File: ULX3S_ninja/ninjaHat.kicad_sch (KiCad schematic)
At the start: 14 parts, among them J1 DVI-HX-107DIP, P1 ULX3S connector (JP1)

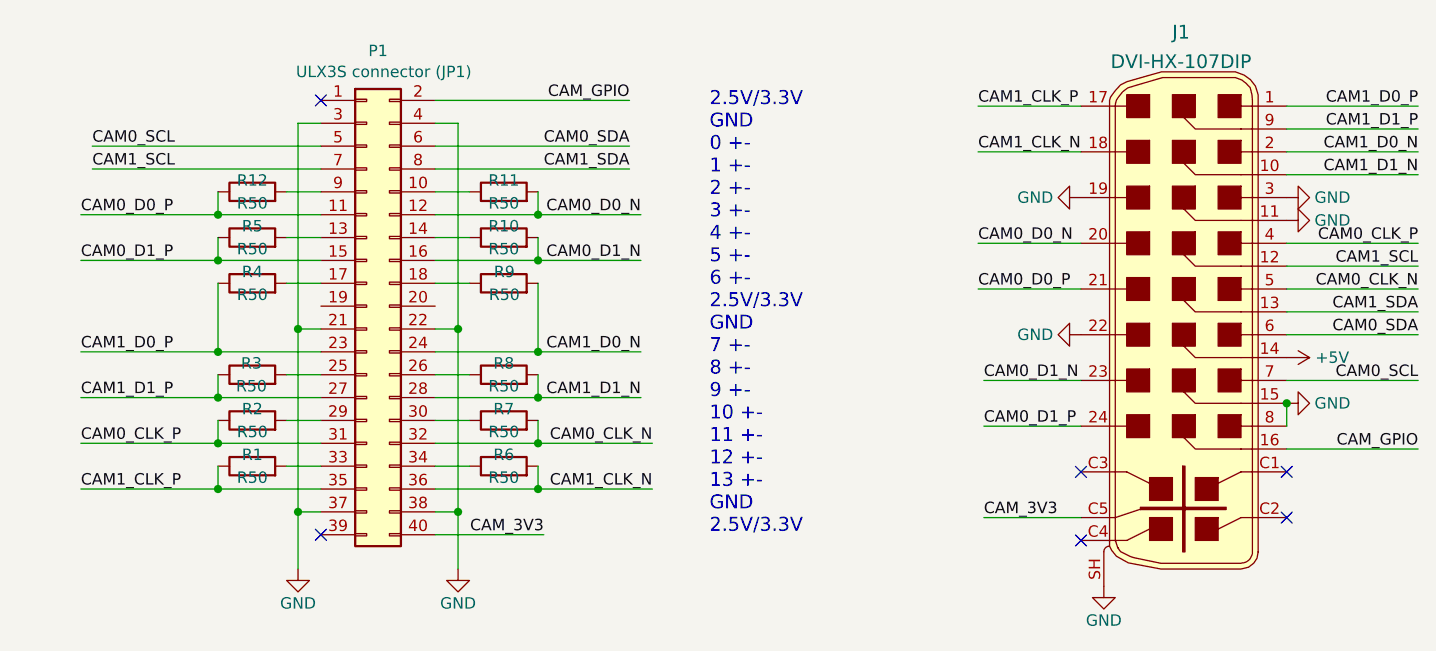
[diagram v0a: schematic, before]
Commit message: Changed circuit
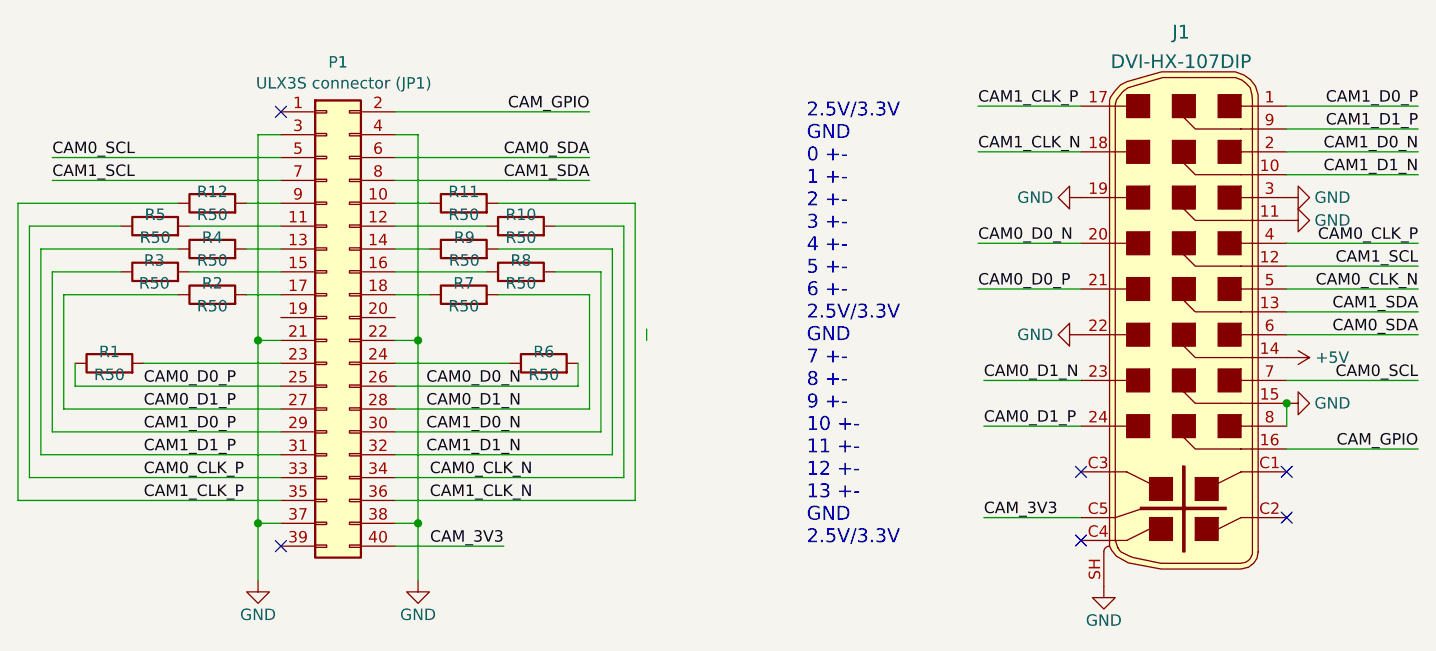
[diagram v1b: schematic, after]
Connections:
- net CAM0_CLK_N: now also P1.34 (Pin_34), R10.2; no longer P1.32 (Pin_32), R7.2
- net CAM0_CLK_P: now also P1.33 (Pin_33), R5.1; no longer P1.31 (Pin_31), R2.1
- net CAM0_D0_N: now also P1.26 (Pin_26), R6.2; no longer P1.12 (Pin_12), R11.2
- net CAM0_D0_P: now also P1.25 (Pin_25), R1.1; no longer P1.11 (Pin_11), R12.1
- net CAM0_D1_N: now also P1.28 (Pin_28), R7.2; no longer P1.16 (Pin_16), R10.2
- net CAM0_D1_P: now also P1.27 (Pin_27), R2.1; no longer P1.15 (Pin_15), R5.1
- net CAM1_CLK_N: now also R11.2; no longer R6.2
- net CAM1_CLK_P: now also R12.1; no longer R1.1
- net CAM1_D0_N: now also P1.30 (Pin_30), R8.2; no longer P1.24 (Pin_24), R9.2
- net CAM1_D0_P: now also P1.29 (Pin_29), R3.1; no longer P1.23 (Pin_23), R4.1
- net CAM1_D1_N: now also P1.32 (Pin_32), R9.2; no longer P1.28 (Pin_28), R8.2
- net CAM1_D1_P: now also P1.31 (Pin_31), R4.1; no longer P1.27 (Pin_27), R3.1
- net at R5.2: now also P1.11 (Pin_11); no longer P1.13 (Pin_13)
- net at R10.1: now also P1.12 (Pin_12); no longer P1.14 (Pin_14)
- net at R4.2: now also P1.13 (Pin_13); no longer P1.17 (Pin_17)
- net at R9.1: now also P1.14 (Pin_14); no longer P1.18 (Pin_18)
- net at R3.2: now also P1.15 (Pin_15); no longer P1.25 (Pin_25)
- net at R8.1: now also P1.16 (Pin_16); no longer P1.26 (Pin_26)
- net at R2.2: now also P1.17 (Pin_17); no longer P1.29 (Pin_29)
- net at R7.1: now also P1.18 (Pin_18); no longer P1.30 (Pin_30)
- net at R1.2: now also P1.23 (Pin_23); no longer P1.33 (Pin_33)
- net at R6.1: now also P1.24 (Pin_24); no longer P1.34 (Pin_34)
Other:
- moved on the sheet: P1, R1, R10, R11, R12, R2, R3, R4, R5, R6, R7, R8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
